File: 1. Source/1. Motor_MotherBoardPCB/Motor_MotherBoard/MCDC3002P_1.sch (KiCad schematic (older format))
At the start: 3 parts, among them U10 CON_6pin_motor, U5 MCDC3002P

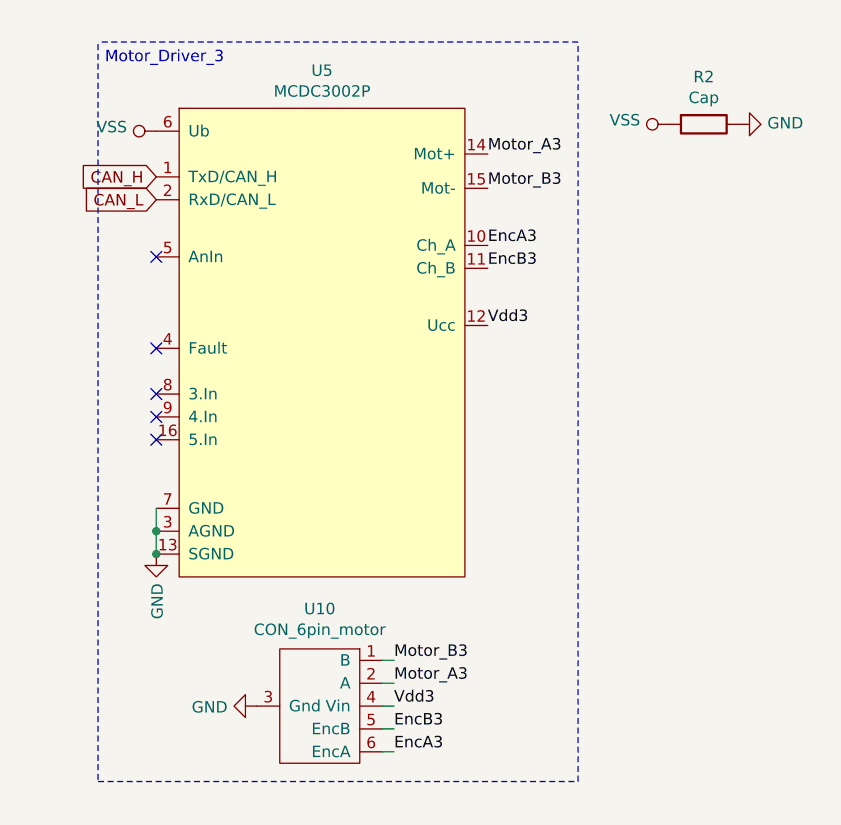
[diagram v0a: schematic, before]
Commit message: PCB_MotorMotherBoard
PCB_MotorMotherBoard
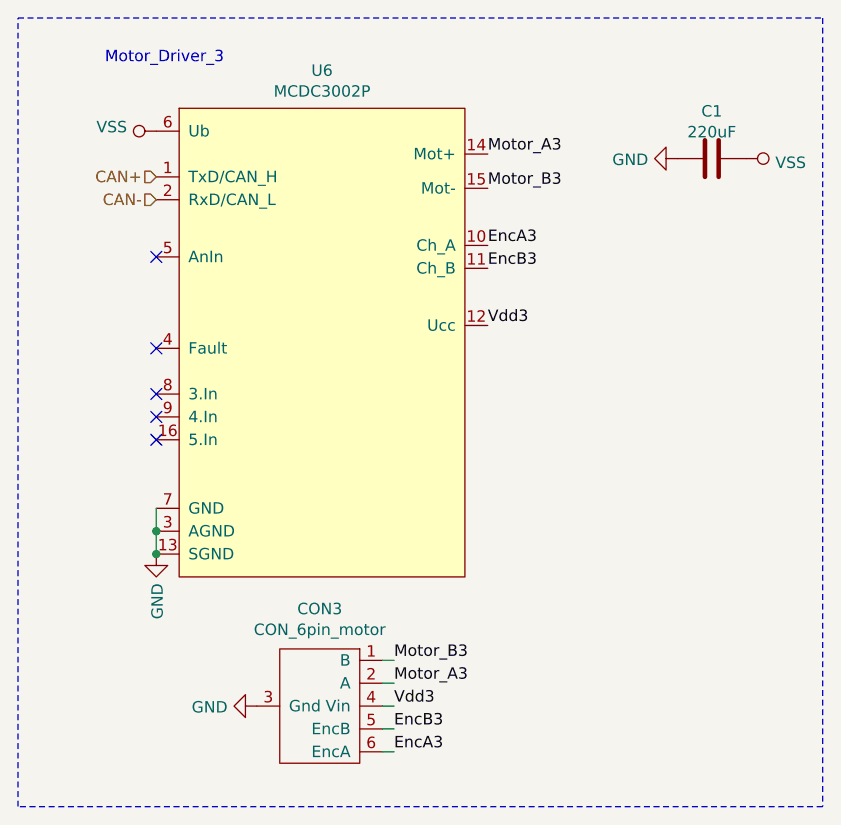
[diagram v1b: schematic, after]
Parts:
- removed R2: Cap, Resistor_THT:R_Axial_DIN0414_L11.9mm_D4.5mm_P5.08mm_Vertical, symbol Device:R
- removed U10: CON_6pin_motor, Connector_IDC:IDC-Header_2x03_P2.54mm_Vertical, symbol BC_Connectors:CON_6pin_motor
- removed U5: MCDC3002P, BC_Motor_Driver:MCDC_3002P, symbol BC_Motor_Drivers:MCDC3002P
- added C1: 220uF, Capacitor_THT:CP_Radial_D8.0mm_P3.50mm, symbol Device:C
- added CON3: CON_6pin_motor, Connector_IDC:IDC-Header_2x03_P2.54mm_Vertical, symbol BC_Connectors:CON_6pin_motor
- added U6: MCDC3002P, BC_Motor_Driver:MCDC_3002P, symbol BC_Motor_Drivers:MCDC3002P
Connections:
- net EncA3: now also CON3.6 (EncA), U6.10 (Ch_A)
- net EncB3: now also CON3.5 (EncB), U6.11 (Ch_B)
- net GND: now also C1.2, CON3.3 (Gnd), U6.13 (SGND), U6.3 (AGND), U6.7 (GND)
- net Motor_A3: now also CON3.2 (A), U6.14 (Mot+)
- net Motor_B3: now also CON3.1 (B), U6.15 (Mot-)
- net VSS: now also C1.1, U6.6 (Ub)
- net Vdd3: now also CON3.4 (Vin), U6.12 (Ucc)
- new net CAN+: U6.1 (TxD/CAN_H)
- new net CAN-: U6.2 (RxD/CAN_L)
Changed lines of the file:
@@
 $EndDescr
 $Comp
-L BC_Motor_Drivers:MCDC3002P U5
-U 1 1 5E4A3DCE
+L BC_Motor_Drivers:MCDC3002P U6
+U 1 1 6362D407
 P 4625 2850
-AR Path="/6360B141/5E4A3DCE" Ref="U5"  Part="1"
-AR Path="/6362A5AD/5E4A3DCE" Ref="U?"  Part="1"
-F 0 "U5" H 4650 4015 50  0000 C CNN
+F 0 "U6" H 4650 4015 50  0000 C CNN
 F 1 "MCDC3002P" H 4650 3924 50  0000 C CNN
 F 2 "BC_Motor_Driver:MCDC_3002P" H 5075 2550 50  0001 C CNN
@@
 $EndComp
 $Comp
-L BC_Connectors:CON_6pin_motor U10
-U 1 1 5E4B2694
+L BC_Connectors:CON_6pin_motor CON3
+U 1 1 6362D408
 P 4665 4465
-AR Path="/6360B141/5E4B2694" Ref="U10"  Part="1"
-AR Path="/6362A5AD/5E4B2694" Ref="U?"  Part="1"
-F 0 "U10" V 4240 4440 50  0000 C CNN
+F 0 "CON3" V 4240 4440 50  0000 C CNN
 F 1 "CON_6pin_motor" V 4331 4440 50  0000 C CNN
 F 2 "Connector_IDC:IDC-Header_2x03_P2.54mm_Vertical" H 4665 4565 50  0001 C CNN
@@
 	4915 4265 4965 4265
 $Comp
-L power:GND #PWR0132
-U 1 1 5E4B26A0
+L power:GND #PWR021
+U 1 1 638358A1
 P 4365 4465
-AR Path="/6360B141/5E4B26A0" Ref="#PWR0132"  Part="1"
-AR Path="/6362A5AD/5E4B26A0" Ref="#PWR?"  Part="1"
-F 0 "#PWR0132" H 4365 4215 50  0001 C CNN
+F 0 "#PWR021" H 4365 4215 50  0001 C CNN
 F 1 "GND" V 4370 4337 50  0000 R CNN
 F 2 "" H 4365 4465 50  0001 C CNN
@@
 	3925 3700 3925 3800
 $Comp
-L power:GND #PWR0133
-U 1 1 5E4B857F
+L power:GND #PWR020
+U 1 1 638358A2
 P 3925 3800
-AR Path="/6360B141/5E4B857F" Ref="#PWR0133"  Part="1"
-AR Path="/6362A5AD/5E4B857F" Ref="#PWR?"  Part="1"
-F 0 "#PWR0133" H 3925 3550 50  0001 C CNN
+F 0 "#PWR020" H 3925 3550 50  0001 C CNN
 F 1 "GND" V 3930 3672 50  0000 R CNN
 F 2 "" H 3925 3800 50  0001 C CNN
@@
 NoConn ~ 3925 3300
 Connection ~ 3925 3800
-Wire Notes Line
-	3670 1570 3670 4795
-Wire Notes Line
-	3670 4795 5770 4795
-Wire Notes Line
-	5770 4795 5770 1560
-Wire Notes Line
-	5770 1560 3670 1560
 Text Notes 3700 1660 0    50   ~ 0
 Motor_Driver_3\n
@@
 Wire Wire Line
 	4915 4365 4965 4365
-Text GLabel 3925 2150 0    50   Input ~ 0
-CAN_H
-Text GLabel 3925 2250 0    50   Input ~ 0
-CAN_L
 $Comp
-L Device:R R?
-U 1 1 6362B9B3
-P 6320 1920
-AR Path="/635EAE14/6362B9B3" Ref="R?"  Part="1"
-AR Path="/6360DF7C/6362B9B3" Ref="R?"  Part="1"
-AR Path="/6360B141/6362B9B3" Ref="R2"  Part="1"
-F 0 "R2" V 6113 1920 50  0000 C CNN
-F 1 "Cap" V 6204 1920 50  0000 C CNN
-F 2 "Resistor_THT:R_Axial_DIN0414_L11.9mm_D4.5mm_P5.08mm_Vertical" V 6250 1920 50  0001 C CNN
-F 3 "~" H 6320 1920 50  0001 C CNN
-	1    6320 1920
+L Device:C R?
+U 1 1 6362C896
+P 6355 2070
+AR Path="/635EAE14/6362C896" Ref="R?"  Part="1"
+AR Path="/6360DF7C/6362C896" Ref="R?"  Part="1"
+AR Path="/6362A5B1/6362C896" Ref="C1"  Part="1"
+AR Path="/6360B141/6362C896" Ref="C1"  Part="1"
+F 0 "C1" V 6148 2070 50  0000 C CNN
+F 1 "220uF" V 6239 2070 50  0000 C CNN
+F 2 "Capacitor_THT:CP_Radial_D8.0mm_P3.50mm" V 6285 2070 50  0001 C CNN
+F 3 "~" H 6355 2070 50  0001 C CNN
+	1    6355 2070
 	0    1    1    0
 $EndComp
 $Comp
 L power:VSS #PWR?
-U 1 1 6362B9B9
-P 6170 1920
-AR Path="/635EAE14/6362B9B9" Ref="#PWR?"  Part="1"
-AR Path="/6360DF7C/6362B9B9" Ref="#PWR?"  Part="1"
-AR Path="/6360B141/6362B9B9" Ref="#PWR015"  Part="1"
-F 0 "#PWR015" H 6170 1770 50  0001 C CNN
-F 1 "VSS" V 6188 2048 50  0000 L CNN
-F 2 "" H 6170 1920 50  0001 C CNN
-F 3 "" H 6170 1920 50  0001 C CNN
-	1    6170 1920
-	0    -1   -1   0
+U 1 1 6362C89C
+P 6505 2070
+AR Path="/635EAE14/6362C89C" Ref="#PWR?"  Part="1"
+AR Path="/6360DF7C/6362C89C" Ref="#PWR?"  Part="1"
+AR Path="/6362A5B1/6362C89C" Ref="#PWR018"  Part="1"
+AR Path="/6360B141/6362C89C" Ref="#PWR018"  Part="1"
+F 0 "#PWR018" H 6505 1920 50  0001 C CNN
+F 1 "VSS" V 6523 2198 50  0000 L CNN
+F 2 "" H 6505 2070 50  0001 C CNN
+F 3 "" H 6505 2070 50  0001 C CNN
+	1    6505 2070
+	0    1    1    0
 $EndComp
 $Comp
 L power:GND #PWR?
-U 1 1 6362B9BF
-P 6470 1920
-AR Path="/635EAE14/6362B9BF" Ref="#PWR?"  Part="1"
-AR Path="/6360DF7C/6362B9BF" Ref="#PWR?"  Part="1"
-AR Path="/6360B141/6362B9BF" Ref="#PWR016"  Part="1"
-F 0 "#PWR016" H 6470 1670 50  0001 C CNN
-F 1 "GND" V 6475 1792 50  0000 R CNN
-F 2 "" H 6470 1920 50  0001 C CNN
-F 3 "" H 6470 1920 50  0001 C CNN
-	1    6470 1920
-	0    -1   -1   0
+U 1 1 6362C8A2
+P 6205 2070
+AR Path="/635EAE14/6362C8A2" Ref="#PWR?"  Part="1"
+AR Path="/6360DF7C/6362C8A2" Ref="#PWR?"  Part="1"
+AR Path="/6362A5B1/6362C8A2" Ref="#PWR019"  Part="1"
+AR Path="/6360B141/6362C8A2" Ref="#PWR019"  Part="1"
+F 0 "#PWR019" H 6205 1820 50  0001 C CNN
+F 1 "GND" V 6210 1942 50  0000 R CNN
+F 2 "" H 6205 2070 50  0001 C CNN
+F 3 "" H 6205 2070 50  0001 C CNN
+	1    6205 2070
+	0    1    1    0
 $EndComp
 $Comp
 L power:VSS #PWR?
-U 1 1 6362BAFC
+U 1 1 6362C93C
 P 3925 1950
-AR Path="/635EAE14/6362BAFC" Ref="#PWR?"  Part="1"
-AR Path="/6360DF7C/6362BAFC" Ref="#PWR?"  Part="1"
-AR Path="/6360B141/6362BAFC" Ref="#PWR014"  Part="1"
-F 0 "#PWR014" H 3925 1800 50  0001 C CNN
+AR Path="/635EAE14/6362C93C" Ref="#PWR?"  Part="1"
+AR Path="/6360DF7C/6362C93C" Ref="#PWR?"  Part="1"
+AR Path="/6362A5B1/6362C93C" Ref="#PWR017"  Part="1"
+AR Path="/6360B141/6362C93C" Ref="#PWR017"  Part="1"
+F 0 "#PWR017" H 3925 1800 50  0001 C CNN
 F 1 "VSS" V 3943 2078 50  0000 L CNN
 F 2 "" H 3925 1950 50  0001 C CNN
@@
 	0    -1   -1   0
 $EndComp
+Text HLabel 3925 2150 0    50   Input ~ 0
+CAN+
+Text HLabel 3925 2250 0    50   Input ~ 0
+CAN-
+Wire Notes Line
+	3320 1455 6840 1455
+Wire Notes Line
+	6840 1455 6840 4905
+Wire Notes Line
+	6840 4905 3320 4905
+Wire Notes Line
+	3320 4905 3320 1455
 $EndSCHEMATC
